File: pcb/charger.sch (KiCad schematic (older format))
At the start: 24 parts, among them J201 Conn_01x02, J202 Conn_01x02, Q201 Q_NMOS_GSD, U201 MP2359, U202 LM358, U203 MAX4377, U204 LM358

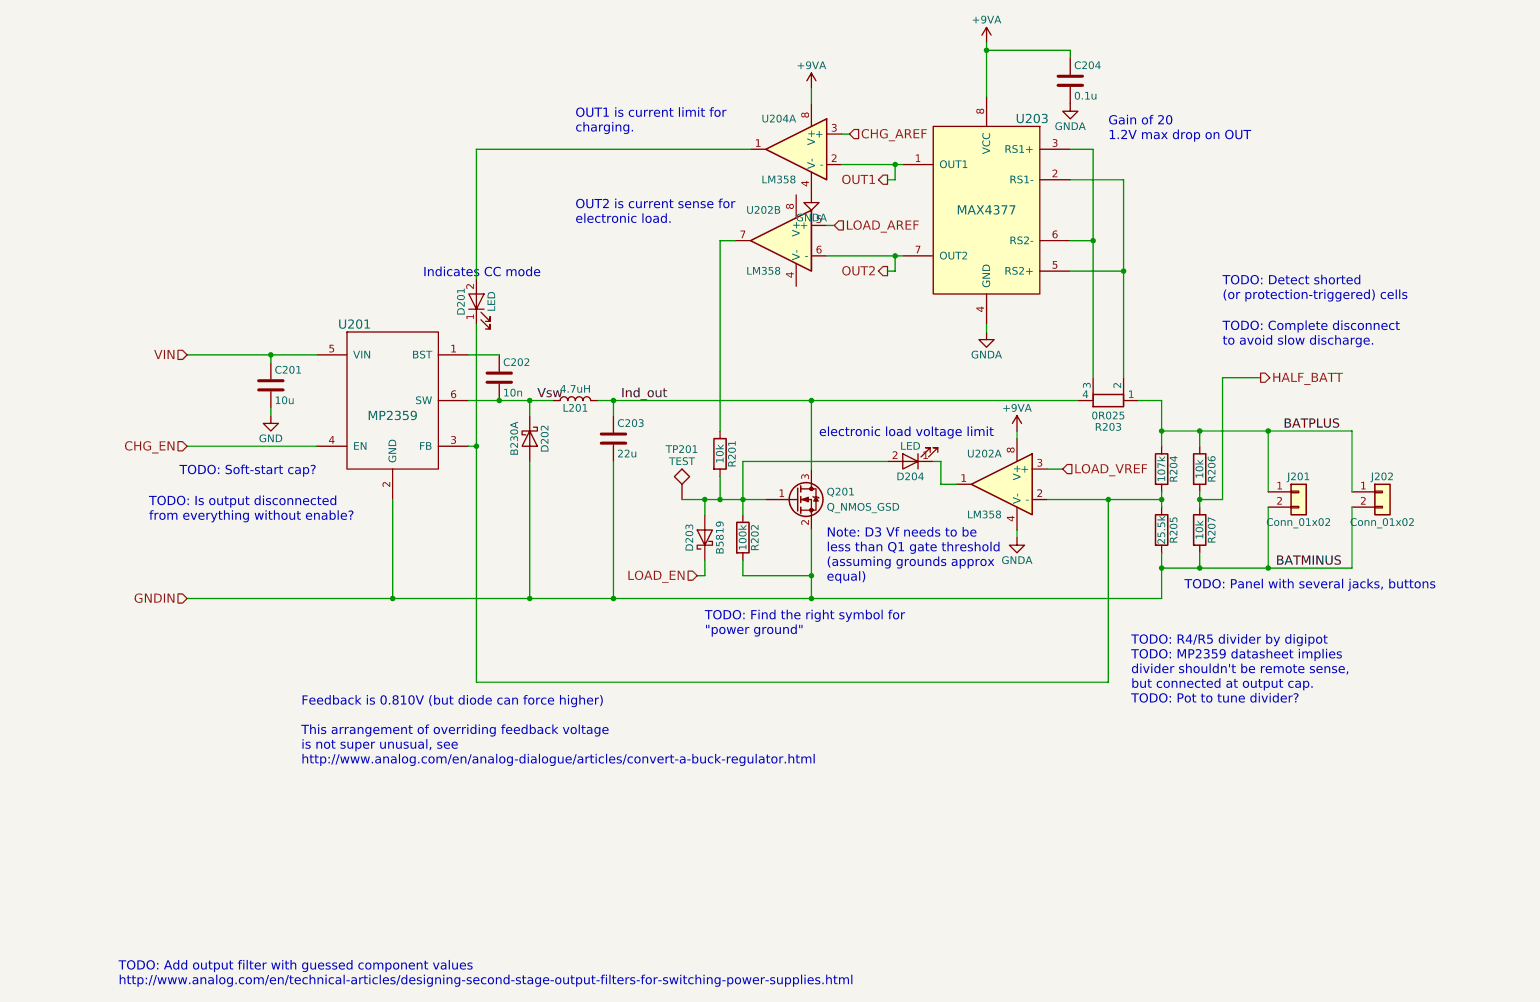
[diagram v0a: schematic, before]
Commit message: Massive rework, fully routed
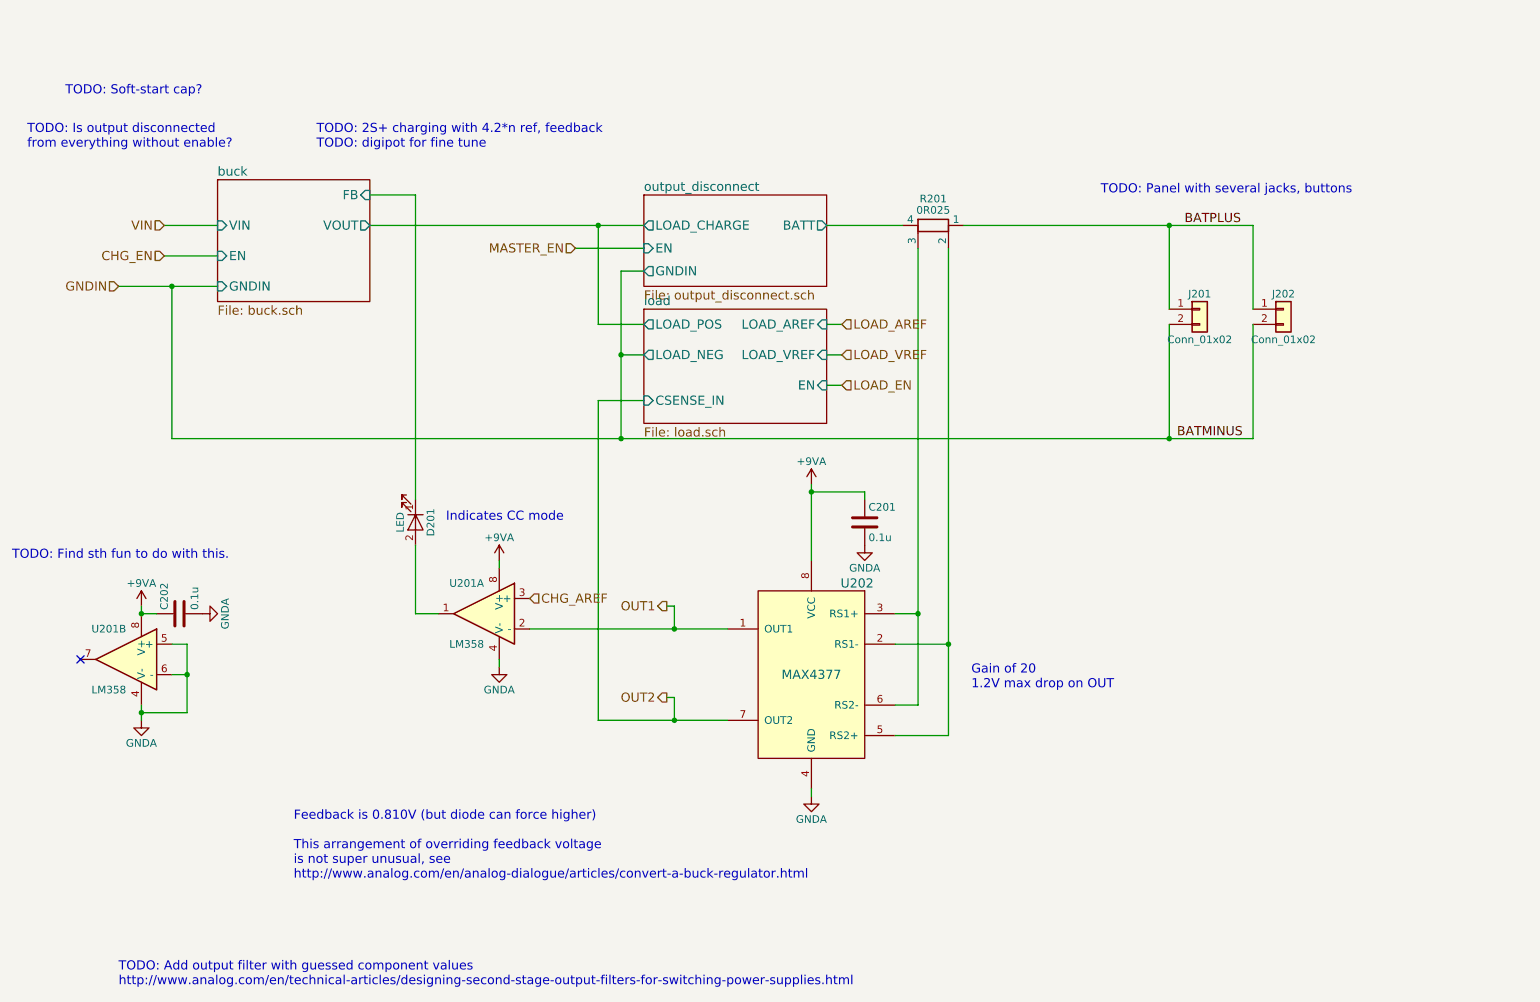
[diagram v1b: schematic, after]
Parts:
- removed C201: 10u, Capacitors_SMD_Round:C_1206, symbol C
- removed C203: 22u, Capacitors_SMD_Round:C_1206, symbol C
- removed D202: B230A, Diodes_SMD:D_SMA, symbol D_Schottky
- removed D203: B5819, Diodes_SMD:D_SOD-323_HandSoldering, symbol D_Schottky
- removed D204: LED, LEDs:LED_0805_HandSoldering, symbol LED
- removed L201: 4.7uH, Inductors_SMD:L_Taiyo-Yuden_NR-50xx, symbol L
- removed Q201: Q_NMOS_GSD, TO_Combo_Packages:TO_220_247, symbol Q_NMOS_GSD
- removed R201, R206, R207: 10k, Resistors_SMD:R_0603_HandSoldering, symbol R
- removed R202: 100k, Resistors_SMD:R_0603_HandSoldering, symbol R
- removed R204: 107k, Resistors_SMD:R_0603_HandSoldering, symbol R
- removed R205: 25.5k, Resistors_SMD:R_0603_HandSoldering, symbol R
- removed TP201: TEST, Measurement_Points:Measurement_Point_Round-SMD-Pad_Small, symbol TEST
- removed U201: MP2359, TO_SOT_Packages_SMD:SOT-23-6_Handsoldering, symbol MP2359
- removed U202: LM358, Housings_SOIC:SOIC-8_3.9x4.9mm_Pitch1.27mm, symbol LM358
- added unit 2 of U201
- C202: value 10n -> 0.1u
- renumbered C204 to C201, R203 to R201, U204 to U201, U203 to U202
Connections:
- net Vsw is gone; now on net GNDA: C202.2
- net +9VA: now also C202.1, U201.8 (V+)
- net GNDA: now also U201.4 (V-), U201.5 (+), U201.6 (-)
- net buck/FB: now reaches D201.1 (K)
- net Ind_out renamed output_disconnect/BATT
- no-connect marks 0 -> 1
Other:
- note added: "TODO: 2S+ charging with 4.2*n ref, feedback\nTODO: digipot for fine tune"
- note added: "TODO: Find sth fun to do with this."
- note removed: "Note: D3 Vf needs to be\nless than Q1 gate threshold\n(assuming grounds approx\nequal)"
- note removed: "OUT1 is current limit for\ncharging."
- note removed: "OUT2 is current sense for\nelectronic load."
- note removed: "TODO: Complete disconnect\nto avoid slow discharge."
- note removed: "TODO: Detect shorted\n(or protection-triggered) cells"
- note removed: "TODO: Find the right symbol for\n"power ground""
- note removed: "TODO: R4/R5 divider by digipot\nTODO: MP2359 datasheet implies\ndivider shouldn't be remote sense,\nbut connected at output cap.\nTODO: Pot to tune divider?"
- note removed: "electronic load voltage limit"
- moved on the sheet: C201, D201, J201, J202, R201, U201A, U202
